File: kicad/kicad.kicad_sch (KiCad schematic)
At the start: 5 parts, among them SW1 SW_Push, SW2 SW_Push, U1 nice_nano, U2 GY-BNO08X, U3 SSD1306_OLED_042

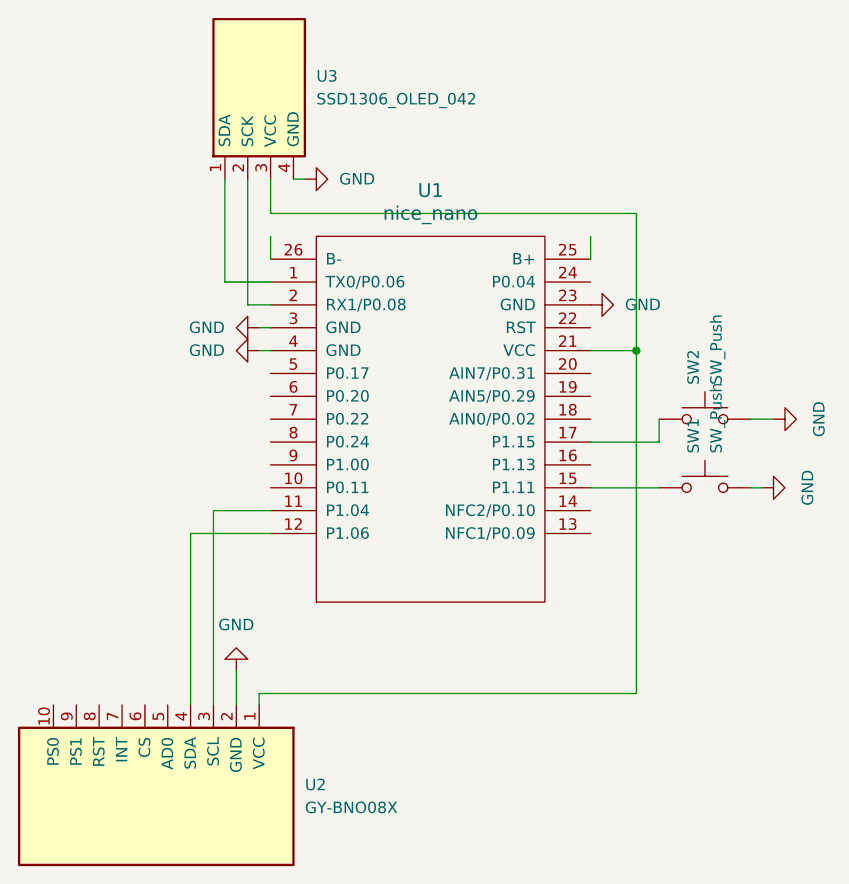
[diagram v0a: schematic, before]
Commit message: kicad cleanup
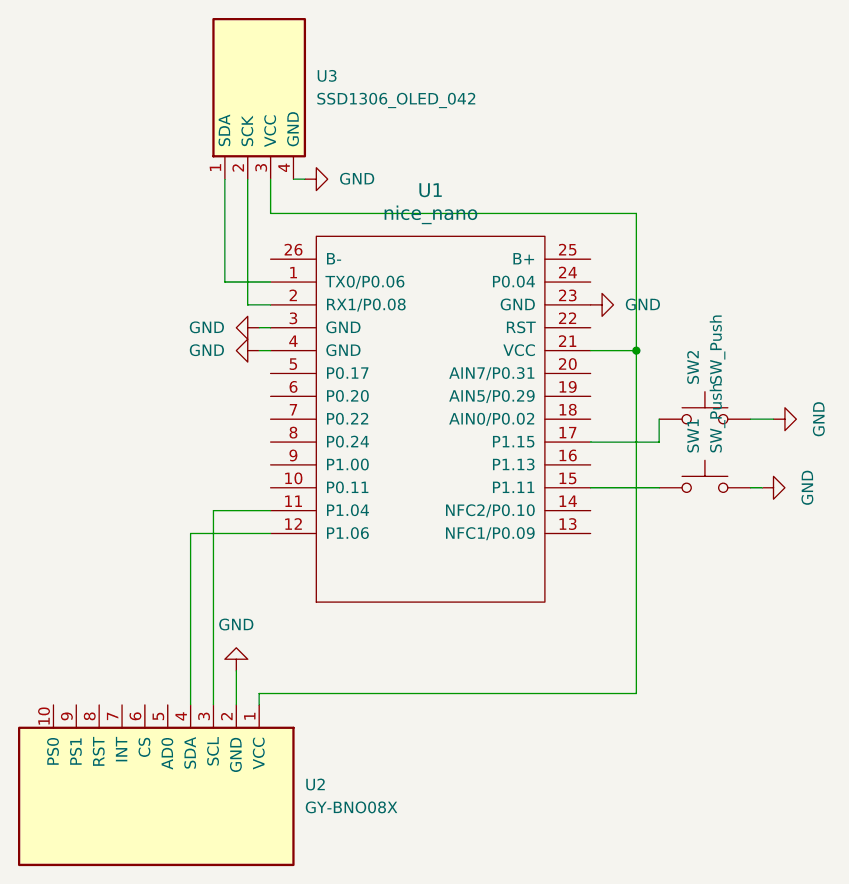
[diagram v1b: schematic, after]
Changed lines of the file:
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@@
-	(wire
-		(pts
-			(xy 104.14 40.64) (xy 104.14 38.1)
-		)
-		(stroke
-			(width 0)
-			(type default)
-		)
-	)
 	(wire
 		(pts
@@
 		)
 		(stroke
-			(width 0)
-			(type default)
-		)
-	)
-	(wire
-		(pts
-			(xy 68.58 38.1) (xy 68.58 40.64)
-		)
-		(stroke
